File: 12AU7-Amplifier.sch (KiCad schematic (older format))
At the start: 31 parts

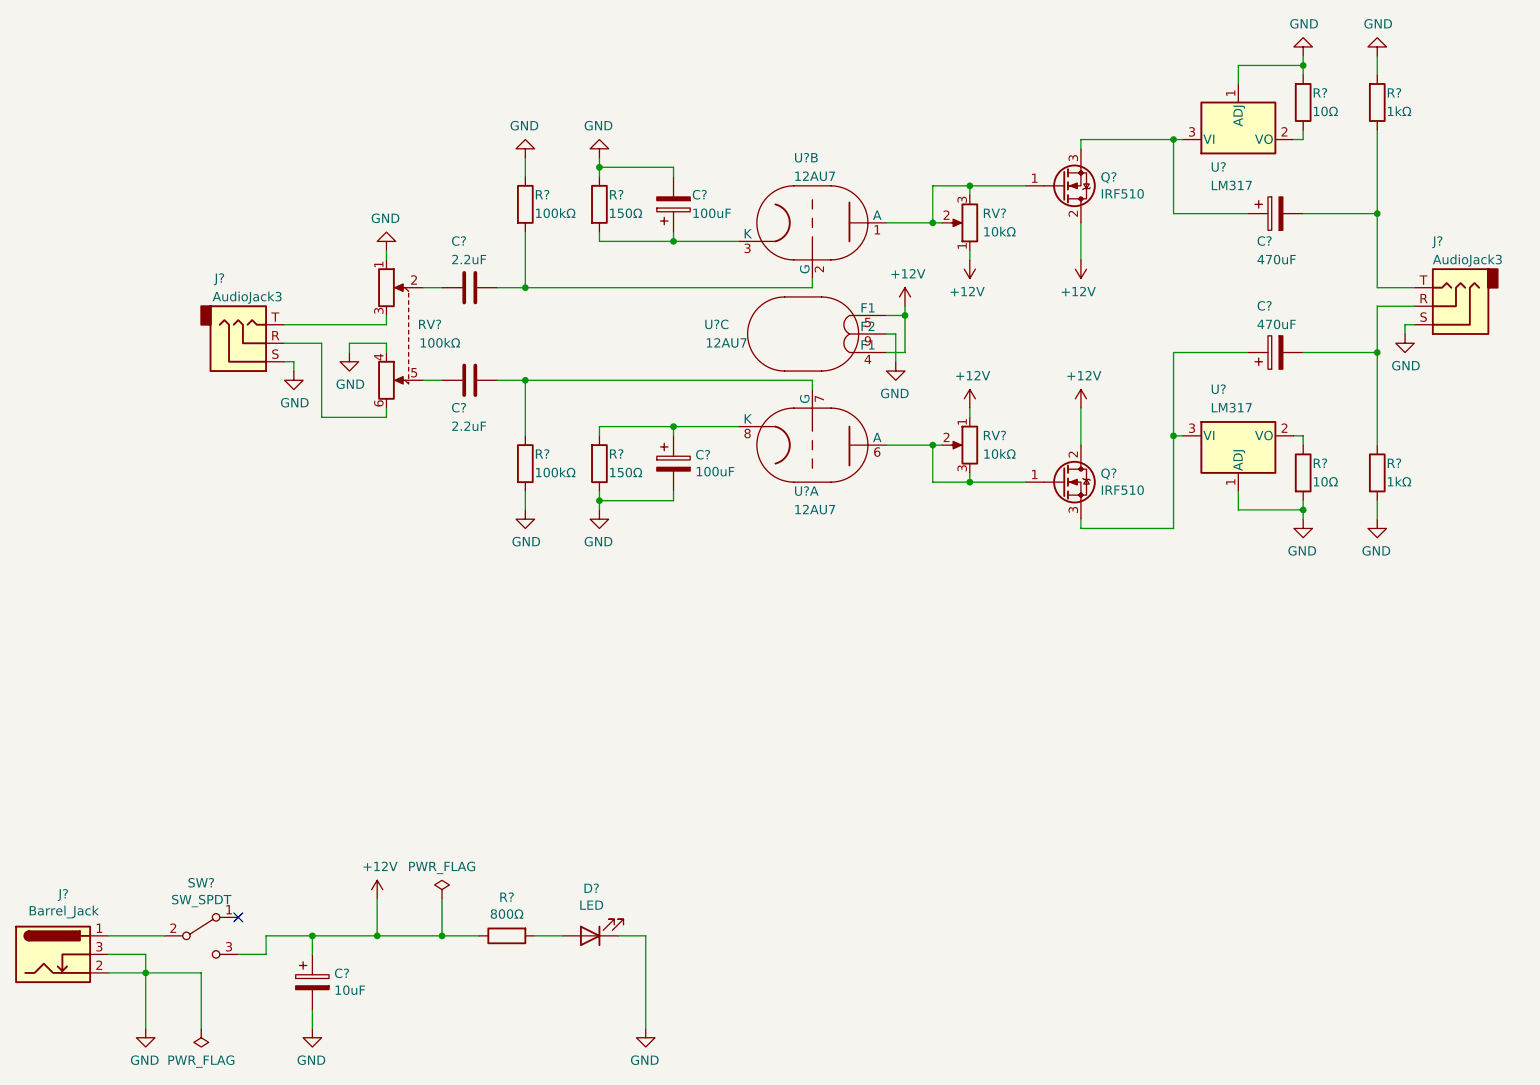
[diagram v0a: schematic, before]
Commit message: Updated page settings
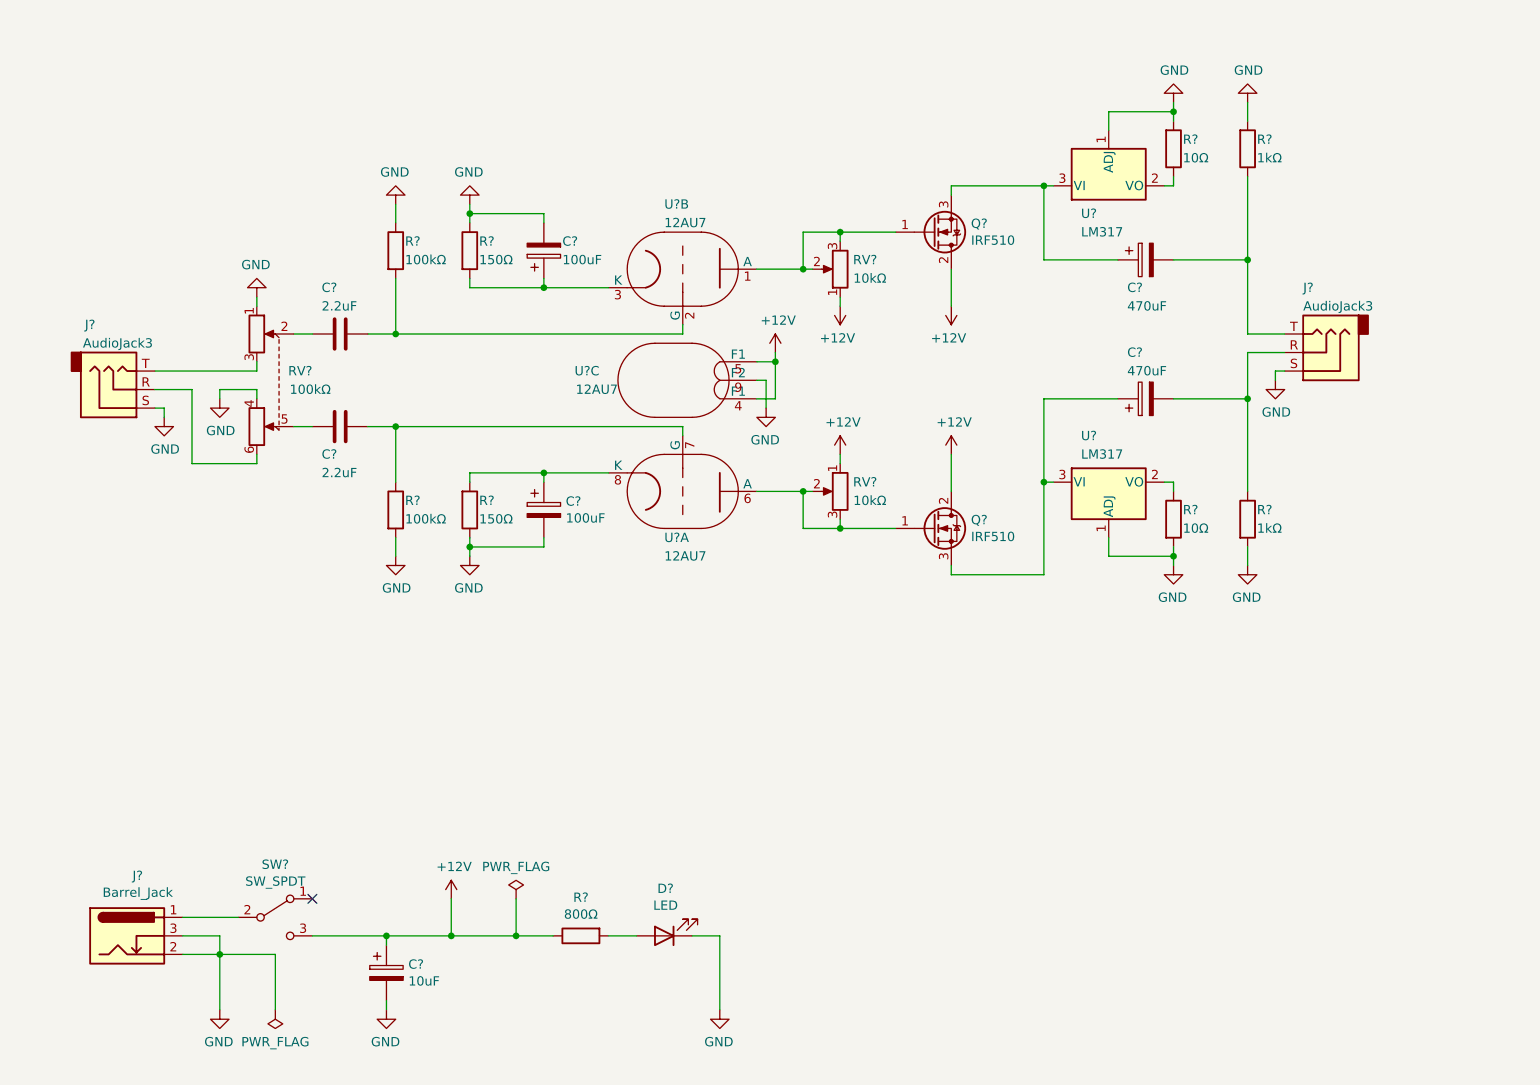
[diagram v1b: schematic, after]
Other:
- moved on the sheet: C?, D?, J?, Q?, R?, RV?, SW?, U?, U?A, U?B, U?C
